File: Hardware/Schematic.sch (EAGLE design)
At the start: 35 parts, among them IC1 XC6220A331MR-G, J1 SAMACSYS_PARTS_USB4110-GF-A, J4 112A-TAAR-R03_ATTEND, Q1 20V/4.2A/52mΩ/1.4W, Q2 SI1308EDL-T1-GE3, U1 ESP32_WROVER_SPARKFUN-IC-POWE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, U2 ESP32-C6-WROOM-1-N8

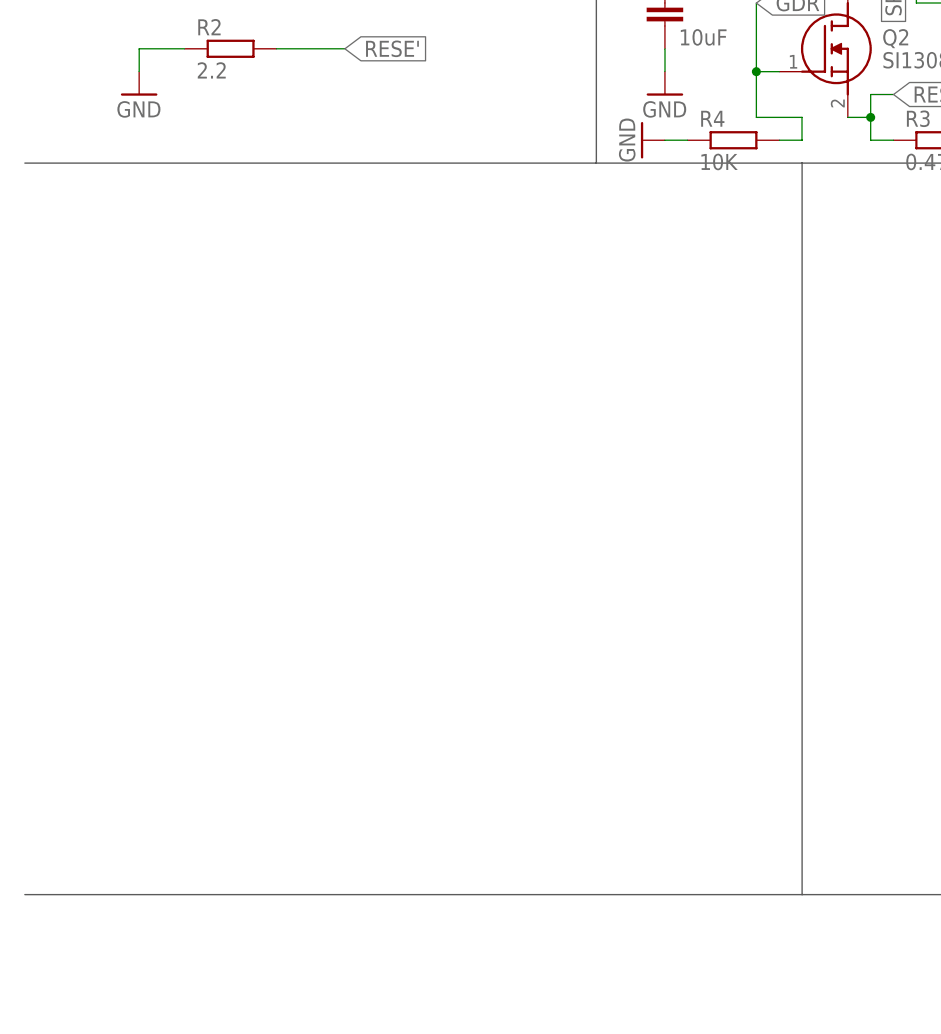
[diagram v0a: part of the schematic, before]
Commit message: add E-Paper Display Header
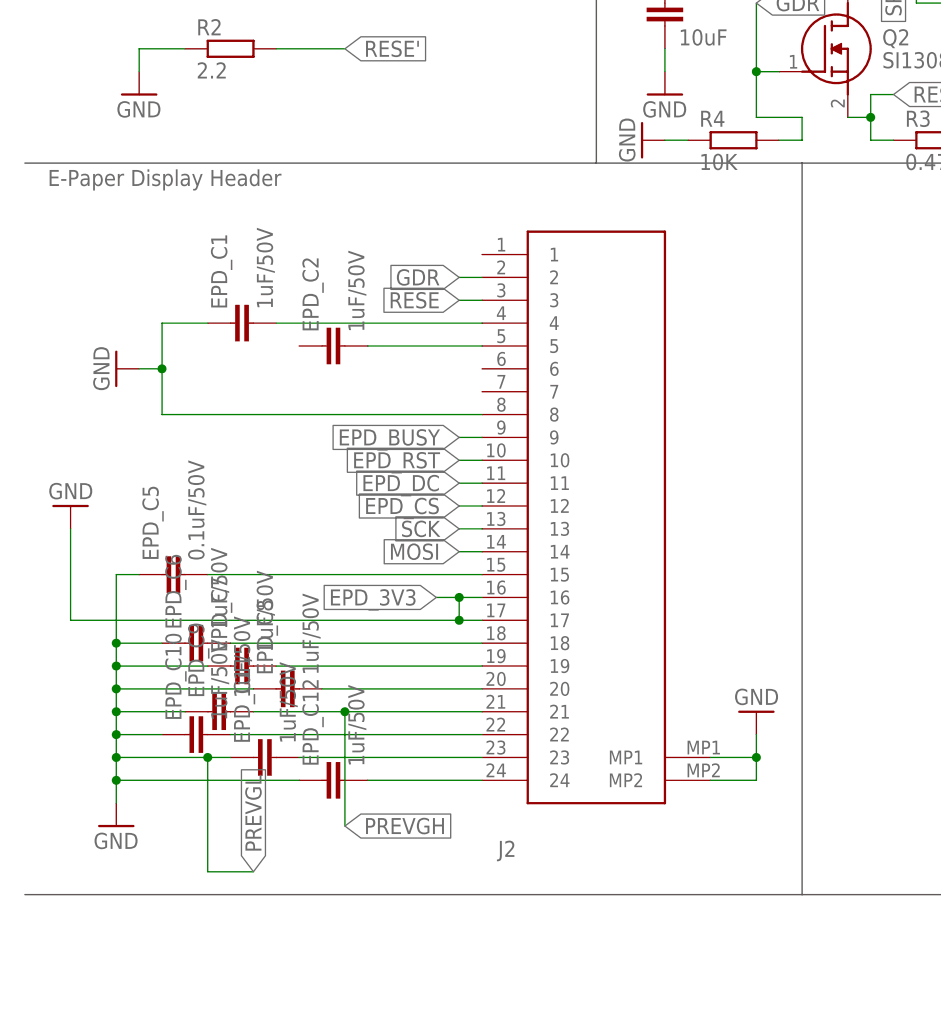
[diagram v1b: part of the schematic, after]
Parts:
- added EPD_C1, EPD_C10, EPD_C11, EPD_C12, EPD_C2, EPD_C6, EPD_C7, EPD_C8, EPD_C9: 1uF/50V, DeskAssistant v19 v1.flbr:EAGLE-LTSPICE_CC0402
- added EPD_C5: 0.1uF/50V, DeskAssistant v19 v1.flbr:EAGLE-LTSPICE_CC0402
- added J2: FH34SRJ-24S-0.5SH_99_, DeskAssistant v19 v1.flbr:FH34SRJ-24S-0.5SH_99_
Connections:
- new net EPD_RST: J2.10
- new net N$10: EPD_C2.2, J2.5
- new net N$11: EPD_C5.2, J2.15
- new net N$12: EPD_C12.2, J2.24
- new net N$13: EPD_C11.2, J2.23
- new net N$14: EPD_C10.2, J2.22
- new net N$16: EPD_C8.2, J2.20
- new net N$17: EPD_C7.2, J2.19
- new net N$18: EPD_C6.2, J2.18
- new net N$9: EPD_C1.2, J2.4
- net EPD_3V3: now also J2.16, J2.17
- net EPD_BUSY: now also J2.9
- net EPD_CS: now also J2.12
- net EPD_DC: now also J2.11
- net GDR: now also J2.2
- net GND: now also EPD_C1.1, J2.8, J2.MP1, J2.MP2
- net MOSI: now also J2.14
- net PREVGH: now also EPD_C9.2, J2.21
- net PREVGL: now also EPD_C10.1, EPD_C11.1, EPD_C12.1, EPD_C5.1, EPD_C6.1, EPD_C7.1, EPD_C8.1, EPD_C9.1
- net RESE: now also J2.3
- net SCK: now also J2.13
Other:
- note added: "E-Paper Display Header"
